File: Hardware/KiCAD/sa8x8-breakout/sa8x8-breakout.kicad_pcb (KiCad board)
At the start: 2 copper layers, 49.6 x 35.6 mm, 11 parts, among them J1 Conn_01x10, J2 Conn_01x10, J3 Conn_Coaxial, J4 Conn_01x07, J5 Conn_01x04, J6 Conn_01x07, U1 SA868

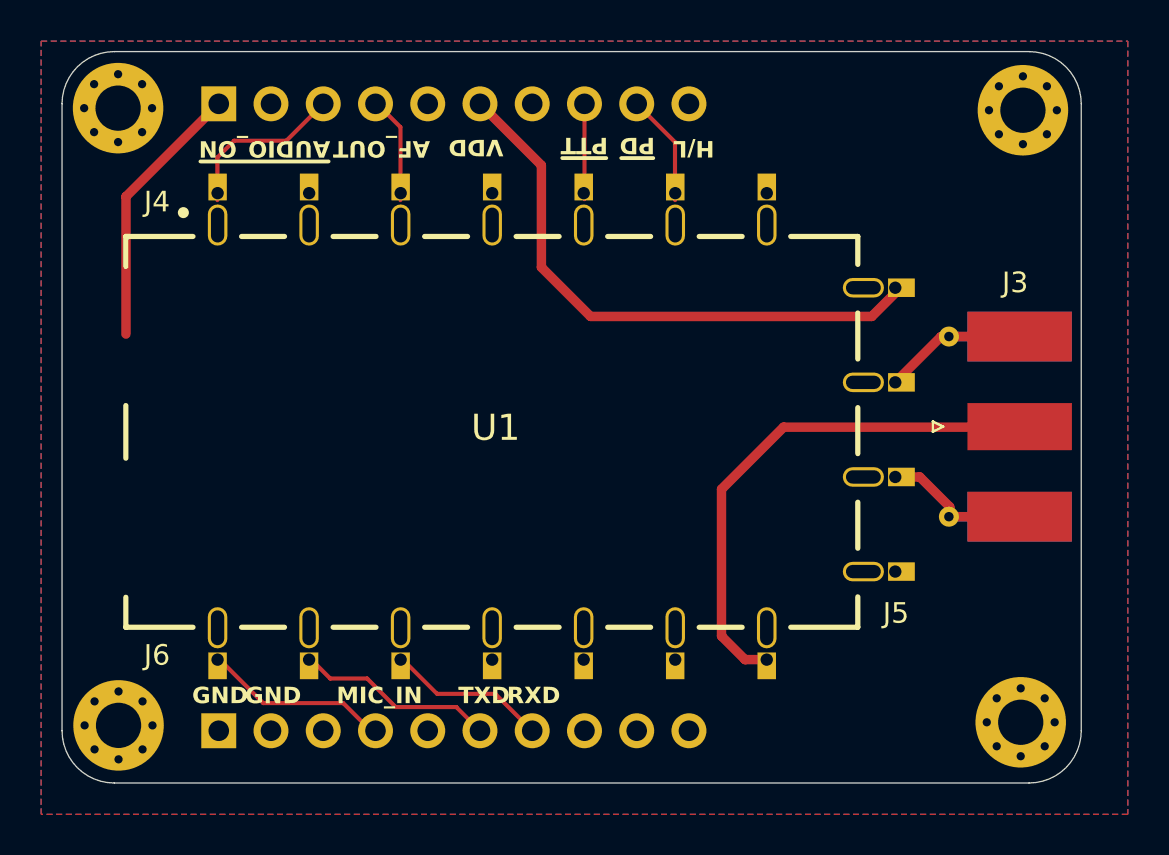
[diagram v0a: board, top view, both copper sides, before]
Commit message: fix: bring sa8x8 flexypins closer, add smps resistor
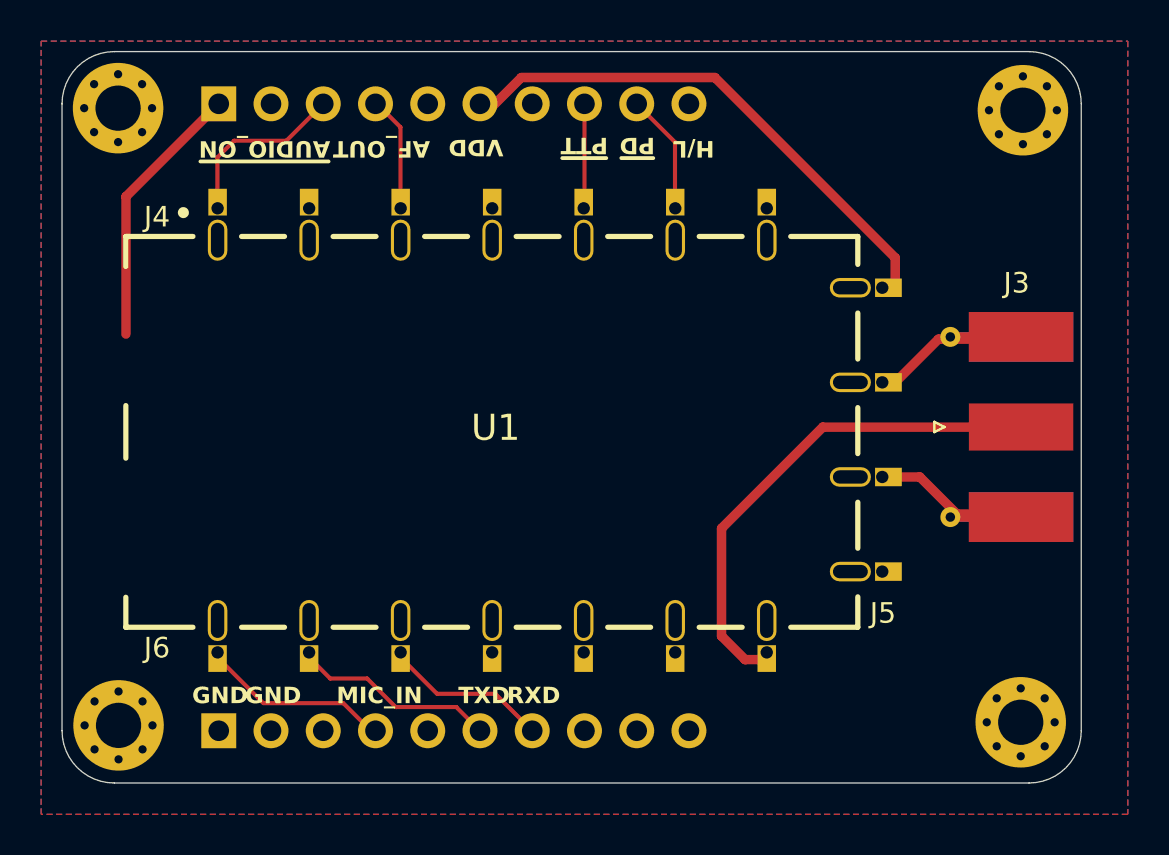
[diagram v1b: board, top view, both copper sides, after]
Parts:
- moved J4 0.74 mm to (163.8, 78.7)
- moved J5 0.63 mm to (169.4, 96.4)
- moved J6 0.35 mm to (137.1, 100.3)
- moved J3 0.07 mm to (174.4, 89.4)
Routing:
- net GND: track 20.8 -> 27.6 mm
- net VDD: track 28.1 -> 26.1 mm
- net /ANT: track 24.8 -> 23.7 mm
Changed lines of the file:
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@@
 		(sheetname "Root")
 		(sheetfile "sa8x8-breakout.kicad_sch")
+		(attr dnp)
 		(fp_line
 			(start -17.798 -9.4401)
@@
 	(footprint "FlexyPin:FlexyPin_1x04_P4.60mm"
 		(layer "F.Cu")
-		(at 170.050534 96.401419 180)
+		(at 169.418 96.401419 180)
 		(property "Reference" "J5"
 			(at -0.033709 -2.022038 0)
@@
 	(footprint "FlexyPin:FlexyPin_1x07_P4.45mm"
 		(layer "F.Cu")
-		(at 163.803844 78.003255 -90)
+		(at 163.803844 78.74 -90)
 		(property "Reference" "J4"
 			(at 0.420719 29.6463 0)
@@
 	(footprint "Connector_Coaxial:SMA_Molex_73251-1153_EdgeMount_Horizontal"
 		(layer "F.Cu")
-		(at 174.377887 89.353425 180)
+		(at 174.448047 89.371581 180)
 		(descr "Molex SMA RF Connectors, Edge Mount, (http://www.molex.com/pdm_docs/sd/732511150_sd.pdf)")
 		(tags "sma edge")
 		(property "Reference" "J3"
-			(at -1.5 7 0)
+			(at -1.5 7 360)
 			(layer "F.SilkS")
 			(effects
@@
 		)
 		(property "Value" "Conn_Coaxial"
-			(at -1.72 -7.11 0)
+			(at -1.72 -7.11 360)
 			(layer "F.Fab")
 			(effects
@@
 		)
 		(fp_text user "${REFERENCE}"
-			(at -1.5 7 0)
+			(at -1.5 7 360)
 			(layer "F.Fab")
 			(effects
@@
 	(footprint "FlexyPin:FlexyPin_1x07_P4.45mm"
 		(layer "F.Cu")
-		(at 137.101526 100.682648 90)
+		(at 137.101526 100.33 90)
 		(property "Reference" "J6"
 			(at 0.216785 -2.9463 180)
@@
 	)
 	(segment
-		(start 137.16 73.66)
-		(end 132.647 78.173)
+		(start 173.046425 93.603425)
+		(end 176.5015 93.603425)
 		(width 0.46)
 		(layer "F.Cu")
@@
 	)
 	(segment
-		(start 132.647 78.173)
-		(end 132.647 84.8532)
+		(start 172.148528 85.103425)
+		(end 170.050534 87.201419)
 		(width 0.46)
 		(layer "F.Cu")
@@
 	(segment
 		(start 171.244419 91.801419)
-		(end 172.700594 93.257594)
+		(end 173.046425 93.603425)
 		(width 0.46)
 		(layer "F.Cu")
@@
 	)
 	(segment
-		(start 173.107887 84.973425)
-		(end 172.278528 84.973425)
+		(start 137.16 73.66)
+		(end 132.647 78.173)
 		(width 0.46)
 		(layer "F.Cu")
@@
 	)
 	(segment
-		(start 172.278528 84.973425)
-		(end 170.050534 87.201419)
+		(start 132.647 78.173)
+		(end 132.647 84.8532)
 		(width 0.46)
 		(layer "F.Cu")
@@
 	)
 	(segment
-		(start 172.700594 93.257594)
-		(end 172.700594 93.761835)
+		(start 170.050534 91.801419)
+		(end 171.244419 91.801419)
 		(width 0.46)
 		(layer "F.Cu")
@@
 	)
 	(segment
-		(start 170.050534 91.801419)
-		(end 171.244419 91.801419)
+		(start 176.5015 85.103425)
+		(end 172.148528 85.103425)
 		(width 0.46)
 		(layer "F.Cu")
@@
 	)
 	(segment
-		(start 149.86 73.66)
-		(end 152.845578 76.645578)
-		(width 0.46)
-		(layer "F.Cu")
-		(net 10)
-	)
-	(segment
-		(start 155.23642 83.99742)
-		(end 168.909396 83.99742)
+		(start 170.050534 81.150534)
+		(end 170.050534 82.601419)
 		(width 0.46)
 		(layer "F.Cu")
@@
 	)
 	(segment
-		(start 170.050534 82.856282)
-		(end 170.050534 82.601419)
+		(start 161.28 72.38)
+		(end 170.050534 81.150534)
 		(width 0.46)
 		(layer "F.Cu")
@@
 	)
 	(segment
-		(start 152.845578 76.645578)
-		(end 152.845578 81.606578)
+		(start 151.869806 72.38)
+		(end 161.28 72.38)
 		(width 0.46)
 		(layer "F.Cu")
@@
 	)
 	(segment
-		(start 168.909396 83.99742)
-		(end 170.050534 82.856282)
+		(start 149.86 73.66)
+		(end 150.224903 74.024903)
 		(width 0.46)
 		(layer "F.Cu")
@@
 	)
 	(segment
-		(start 152.845578 81.606578)
-		(end 155.23642 83.99742)
+		(start 150.224903 74.024903)
+		(end 151.869806 72.38)
 		(width 0.46)
 		(layer "F.Cu")
@@
 	)
 	(segment
-		(start 162.749633 100.682648)
-		(end 161.603434 99.536449)
+		(start 161.603434 99.536449)
+		(end 161.603434 94.301566)
 		(width 0.46)
 		(layer "F.Cu")
@@
 	)
 	(segment
-		(start 161.603434 99.536449)
-		(end 161.603434 92.396566)
+		(start 162.749633 100.682648)
+		(end 161.603434 99.536449)
 		(width 0.46)
 		(layer "F.Cu")
@@
 	)
 	(segment
-		(start 161.603434 92.396566)
-		(end 164.621599 89.378401)
+		(start 163.801526 100.682648)
+		(end 162.749633 100.682648)
 		(width 0.46)
 		(layer "F.Cu")
@@
 	)
 	(segment
-		(start 164.621599 89.378401)
+		(start 166.526599 89.378401)
 		(end 175.349114 89.378401)
 		(width 0.46)
@@
 	)
 	(segment
-		(start 163.801526 100.682648)
-		(end 162.749633 100.682648)
+		(start 161.603434 94.301566)
+		(end 166.526599 89.378401)
 		(width 0.46)
 		(layer "F.Cu")
